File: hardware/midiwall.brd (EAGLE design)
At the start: 80.7 x 36.8 mm, 25 parts, among them IC1 PIC16F1825SO14

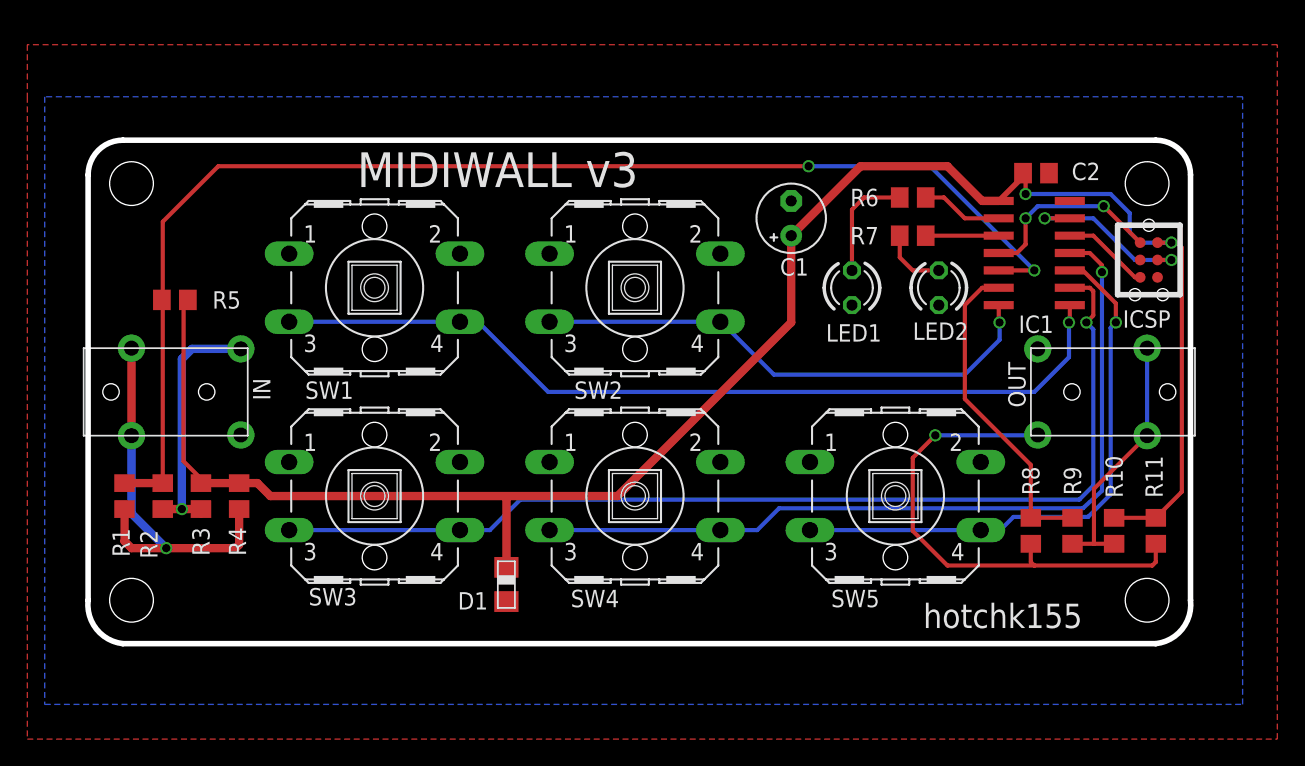
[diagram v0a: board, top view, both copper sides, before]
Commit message: ewr
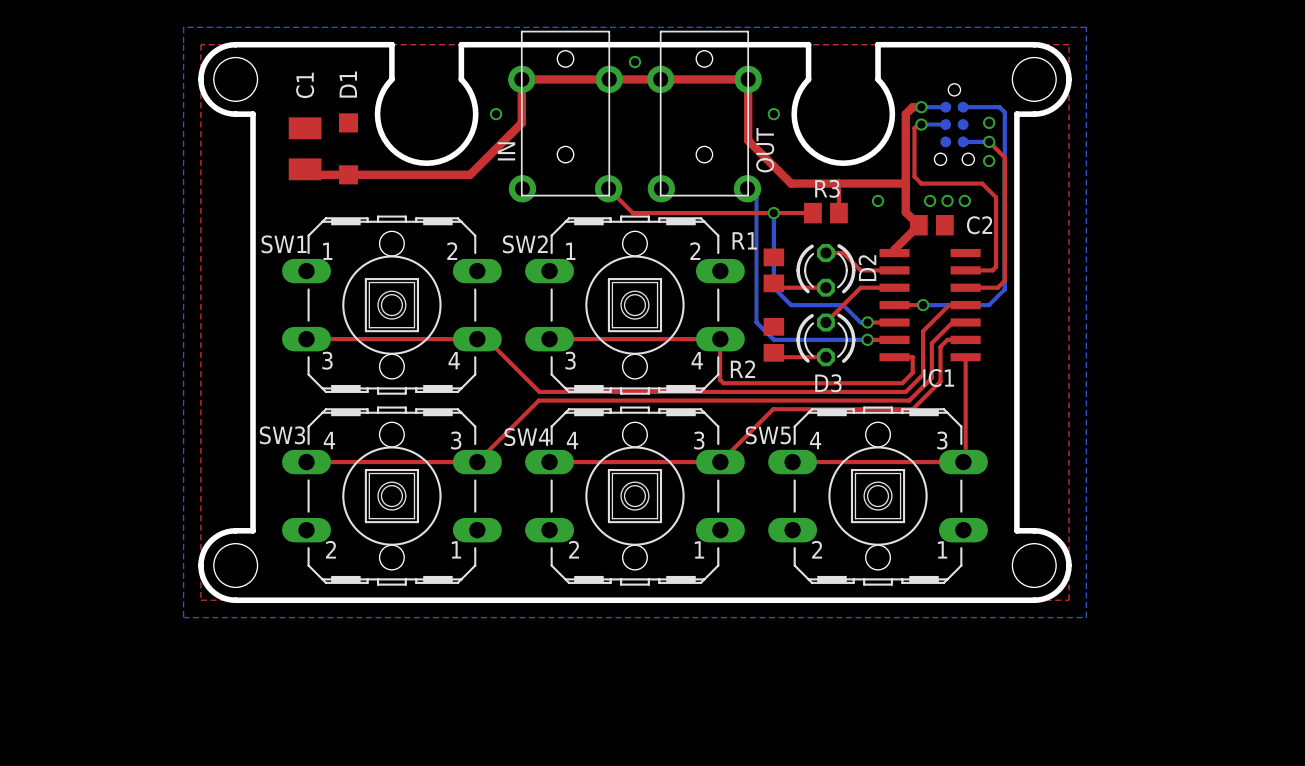
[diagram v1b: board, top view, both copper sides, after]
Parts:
- removed LED1, LED2: (no value), led:LED3MM
- removed R10, R11, R4, R6, R7, R8, R9: (no value), rcl:R0805
- removed R5: 4k7, rcl:R0805
- added D2, D3: (no value), led:LED3MM
- C1: device rcl:E2,5-5 -> resistor:SMC_B
- D1: value 0805DIODE -> MBR0520LT; device jasons_stuff:0805DIODE -> diode:SOD123
- R3: value (none) -> 4k7
- moved R1 50.3 mm to (50.8, 26.7)
- moved R3 50.2 mm to (54.6, 30.9), turned to 0 degrees
- moved R2 46.1 mm to (50.8, 21.6)
- moved OUT 39.6 mm to (45.7, 40.6), turned to 0 degrees
- moved IN 39.1 mm to (35.6, 40.6), turned to 0 degrees
- moved C1 35.9 mm to (16.5, 35.6)
- moved D1 33.9 mm to (19.7, 35.6), turned to 90 degrees
- moved ICSP 17.3 mm to (64.0, 39.9), flipped to the bottom
- moved C2 8.52 mm to (62.4, 30.0)
- moved IC1 8.52 mm to (62.2, 24.1)
- moved SW1 1.80 mm to (22.9, 24.1)
- moved SW2 1.27 mm to (40.6, 24.1)
- moved SW3 1.27 mm to (22.9, 10.2), turned to 180 degrees
- moved SW5 1.27 mm to (58.4, 10.2), turned to 180 degrees
- turned SW4 to 180 degrees
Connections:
- removed net N$5: OUT.3, R11.1, R8.2
- removed net N$7: IN.2, IN.2A, R1.2, R4.1
- removed net N$8: OUT.2, OUT.2A, R10.1, R9.2
- removed net N$9: IN.3, R2.2, R3.1
- net +5V: now also D1.C, IN.2, IN.2A, OUT.2, OUT.2A; no longer D1.A, R10.2, R11.2, R4.2, R5.2
- net GND: now also D1.A, R1.1, R2.1; no longer D1.C, LED1.K, LED2.K
- net KEY1: now also IC1.10; no longer IC1.9
- net KEY3: now also IC1.9; no longer IC1.11
- net KEY4: now also IC1.11; no longer IC1.8
- net KEY5: now also IC1.8; no longer IC1.10
- net LED1: now also D2.A; no longer R6.2
- net LED2: now also D3.A; no longer R7.2
- net N$1: now also D2.K, R1.2; no longer LED1.A, R6.1
- net N$2: now also D3.K, R2.2; no longer LED2.A, R7.1
- net RX: now also IN.3, R3.1; no longer R1.1, R2.1, R5.1
- net TX: now also OUT.3; no longer R8.1, R9.1
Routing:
- net +5V: track 135.7 -> 71.8 mm, vias 2 -> 1
- net RX: track 93.2 -> 31.0 mm
- net N$5: track 37.1 -> 0.00 mm, vias 1 -> 0
- net N$7: track 29.3 -> 0.00 mm, vias 1 -> 0
- net KEY3: track 60.8 -> 35.6 mm, vias 1 -> 0
- net KEY1: track 76.6 -> 53.9 mm, vias 1 -> 0
- net KEY5: track 41.6 -> 20.2 mm, vias 1 -> 0
- net N$8: track 19.0 -> 0.00 mm
- net N$9: track 18.9 -> 0.00 mm, vias 1 -> 0
- net VPP: track 14.0 -> 24.7 mm, vias 2 -> 1
- net KEY4: track 64.1 -> 54.3 mm, vias 1 -> 0
- net PGC: track 6.41 -> 15.6 mm, vias 0 -> 1
- net PGD: track 13.4 -> 20.0 mm, vias 2 -> 1
- net KEY2: track 38.1 -> 32.5 mm, vias 1 -> 0
- net N$1: track 8.31 -> 3.94 mm
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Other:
- board size 80.7 x 36.8 mm -> 63.5 x 40.6 mm
- board text removed: "MIDIWALL v3"
- board text removed: "hotchk155"
